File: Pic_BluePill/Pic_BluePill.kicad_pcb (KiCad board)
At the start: 2 copper layers, 53.2 x 18.2 mm, 27 parts, among them J1 Conn_01x14_Male, J2 USB_B_Micro, J3 Conn_01x14_Male, SW2 SW_Push, U1 LM78L05, U2 PIC18F2550-ISO, Y1 Crystal

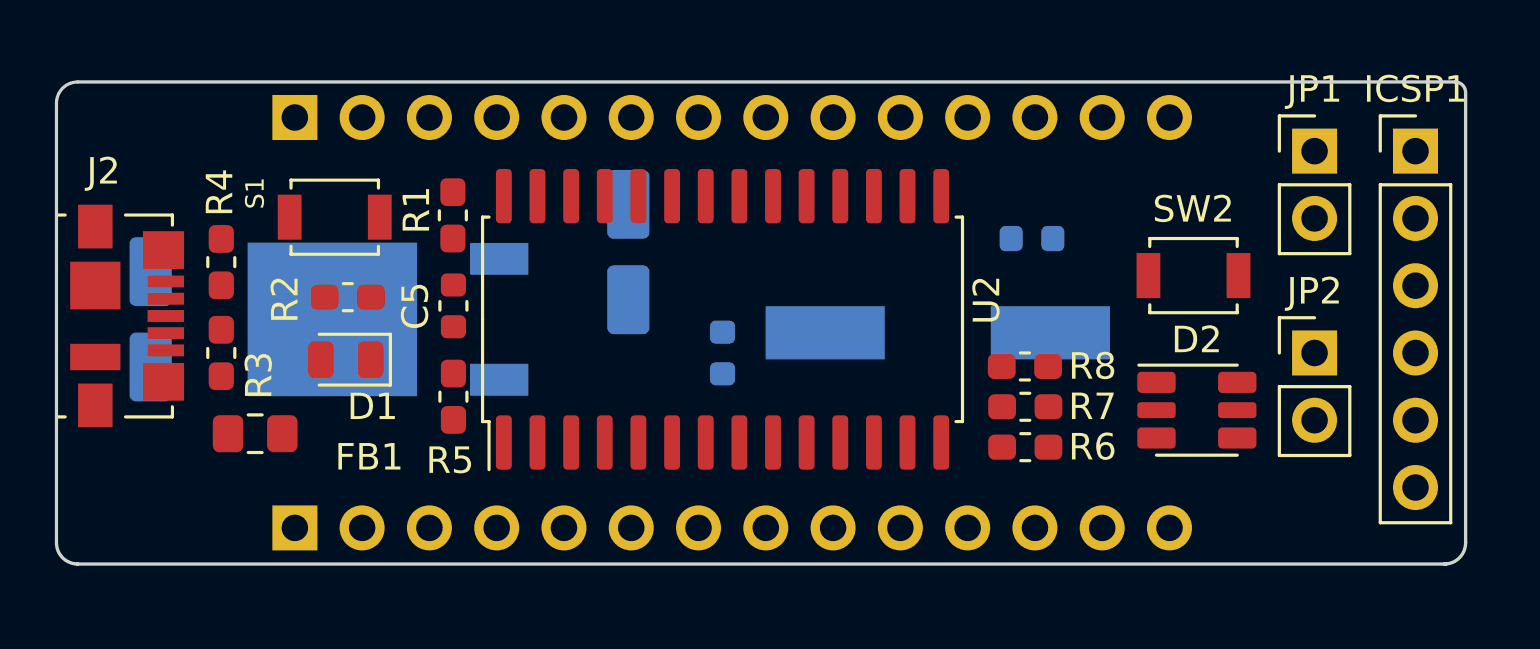
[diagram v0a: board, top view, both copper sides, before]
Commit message: Finalização da Placa - sem arquivos de fabricação
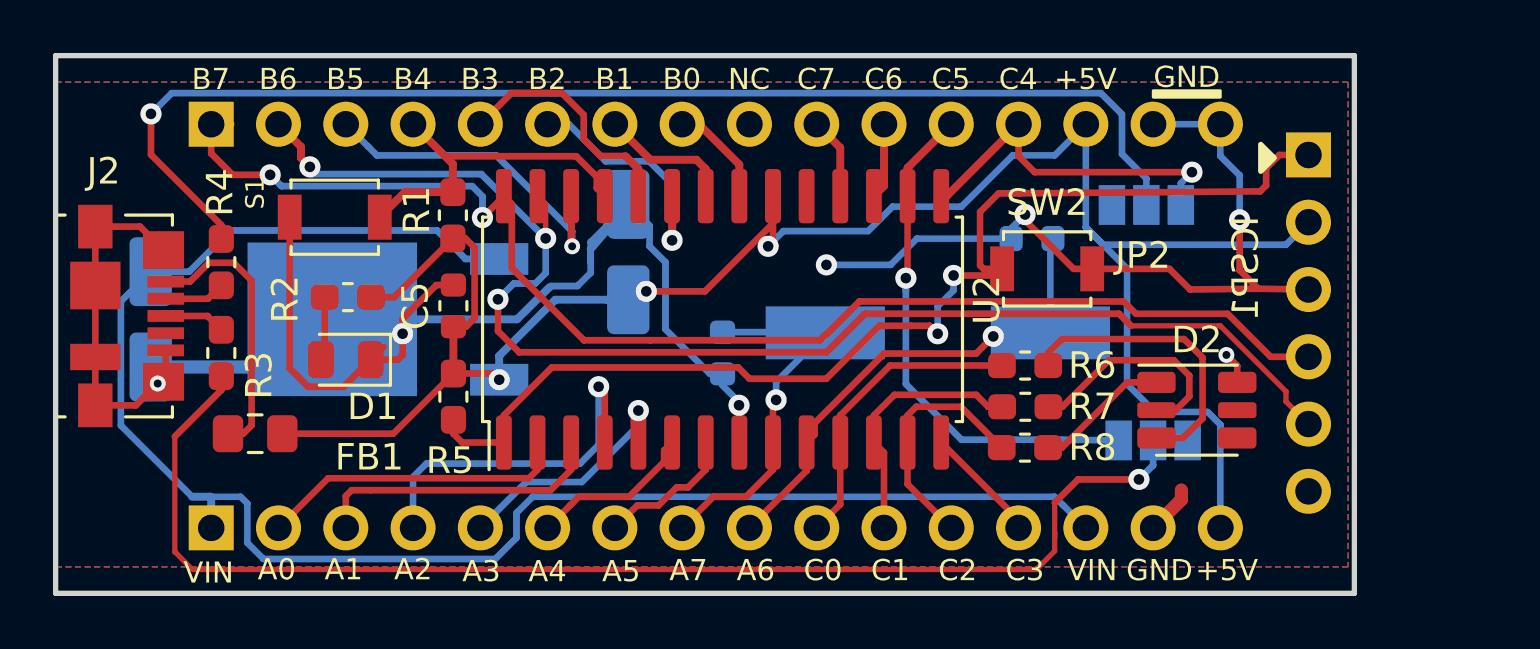
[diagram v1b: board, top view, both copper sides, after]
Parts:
- ICSP1: moved to B.Cu
- J1, J3: value Conn_01x14_Male -> Conn_01x16_Male; footprint Connector_PinHeader_2.54mm:PinHeader_1x14_P2.54mm_Vertical -> Connector_PinHeader_2.54mm:PinHeader_1x16_P2.54mm_Vertical
- JP1, JP2: footprint Connector_PinHeader_2.54mm:PinHeader_1x02_P2.54mm_Vertical -> Jumper:SolderJumper-3_P1.3mm_Open_Pad1.0x1.5mm_NumberLabels; moved to B.Cu
- X1: renamed from Y1; value Crystal -> 20Mhz
- moved JP1 12.5 mm to (168.4, 81.5)
- moved JP2 8.46 mm to (168.1, 72.6), turned to 180 degrees
- moved SW2 5.53 mm to (164.4, 75.1)
- moved ICSP1 4.04 mm to (174.3, 70.8), turned to 180 degrees
- moved J3 3.17 mm to (132.8, 69.6)
- moved J1 3.16 mm to (132.8, 84.8)
- moved R6 3.08 mm to (163.6, 78.7)
- moved R8 3.07 mm to (163.6, 81.8)
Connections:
- C1 pad 1: Net-(C1-Pad1) -> /VIN
- ICSP1 pad 1: Net-(ICSP1-Pad1) -> /VPP
- ICSP1 pad 2: Net-(ICSP1-Pad2) -> +5V
- ICSP1 pad 3: Net-(ICSP1-Pad3) -> GNDREF
- ICSP1 pad 4: Net-(ICSP1-Pad4) -> /B7
- ICSP1 pad 5: Net-(ICSP1-Pad5) -> /B6
- J1 pad 1: /A0 -> /VIN
- J1 pad 10: /OSC.2 -> /C0
- J1 pad 11: /C0 -> /C1
- J1 pad 12: /C1 -> /C2
- J1 pad 13: /C2 -> /C3
- J1 pad 14: /C3 -> /VIN
- J1 pad 2: /A1 -> /A0
- J1 pad 3: /A2 -> /A1
- J1 pad 4: /A3 -> /A2
- J1 pad 5: /A4 -> /A3
- J1 pad 6: /A5 -> /A4
- J1 pad 7: /OSC.1 -> /A5
- J1 pad 8: GNDREF -> /OSC.1
- J1 pad 9: /OSC.1 -> /OSC.2
- J3 pad 10: GNDREF -> /C7
- J3 pad 11: /C7 -> /C6
- J3 pad 12: /C6 -> /C5
- J3 pad 13: /C5 -> /C4
- J3 pad 14: /C4 -> +5V
- J3 pad 9: +5V -> Net-(J3-Pad9)
- R2 pad 2: Net-(R2-Pad2) -> +5V
- U1 pad 1: Net-(C1-Pad1) -> /VIN
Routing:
- net GNDREF: track 0.00 -> 97.0 mm, vias 0 -> 7
- net +5V: track 0.00 -> 76.5 mm, vias 0 -> 3
- net /VIN: track 0.00 -> 63.8 mm
- net /B6: track 0.00 -> 52.3 mm, vias 0 -> 3
- net /B7: track 0.00 -> 50.3 mm, vias 0 -> 2
- net Net-(JP1-Pad2): track 0.00 -> 48.3 mm, vias 0 -> 1
- net Net-(JP2-Pad2): track 0.00 -> 46.9 mm, vias 0 -> 1
- net /VPP: track 0.00 -> 42.6 mm, vias 0 -> 2
- net /C5: track 0.00 -> 20.1 mm, vias 0 -> 1
- net /OSC.2: track 0.00 -> 16.7 mm, vias 0 -> 1
- net /B4: track 0.00 -> 16.6 mm
- net /B5: track 0.00 -> 14.5 mm, vias 0 -> 1
- net /OSC.1: track 0.00 -> 14.4 mm, vias 0 -> 1
- net /A2: track 0.00 -> 13.8 mm, vias 0 -> 1
- net /C4: track 0.00 -> 13.5 mm, vias 0 -> 1
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- added copper zone on B.Cu, net GNDREF
- added copper zone on F.Cu, net GNDREF
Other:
- board size 53.2 x 18.2 mm -> 49 x 20.3 mm
- net class Default: clearance 0.2 -> 0.127
- rule trace_clearance: 0.2 -> 0.127
- board text added: "+5V"
- board text added: "A0"
- board text added: "A1"
- board text added: "A2"
- board text added: "A3"
- board text added: "A4"
- board text added: "A5"
- board text added: "A6"
- board text added: "A7"
- board text added: "B0"
- board text added: "B1"
- board text added: "B2"
- board text added: "B3"
- board text added: "B4"
- board text added: "B5"
- board text added: "B6"
- board text added: "B7"
- board text added: "C0"
- board text added: "C1"
- board text added: "C2"
- board text added: "C3"
- board text added: "C4"
- board text added: "C5"
- board text added: "C6"
- board text added: "C7"
- board text added: "GND"
- board text added: "NC"
- board text added: "Rev. 1.0"
- board text added: "VIN"
